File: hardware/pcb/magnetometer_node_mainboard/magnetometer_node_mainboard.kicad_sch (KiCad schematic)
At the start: 0 parts

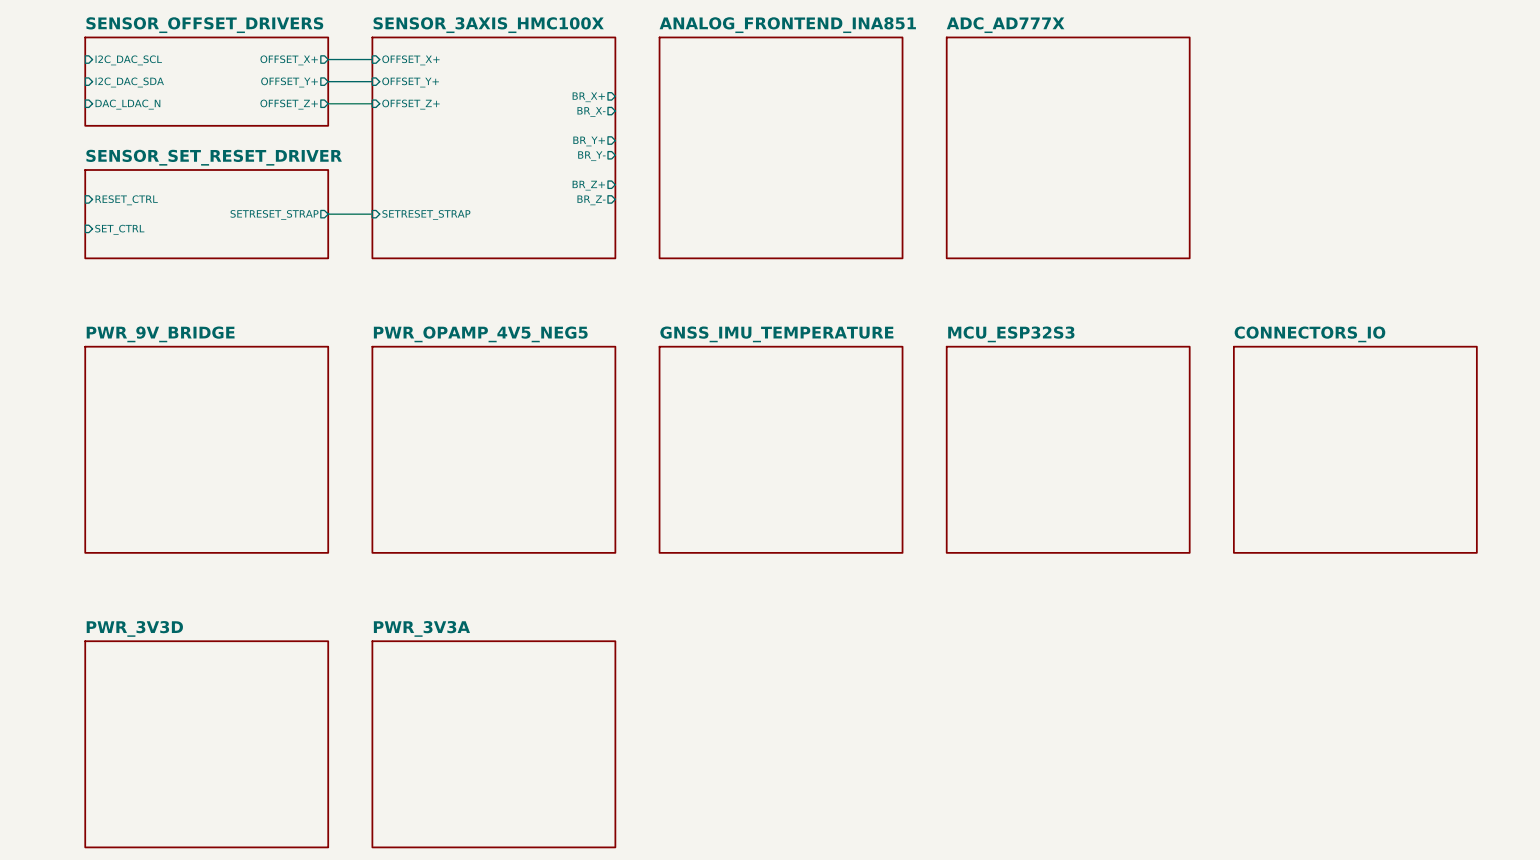
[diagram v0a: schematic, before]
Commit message: first code for the v1
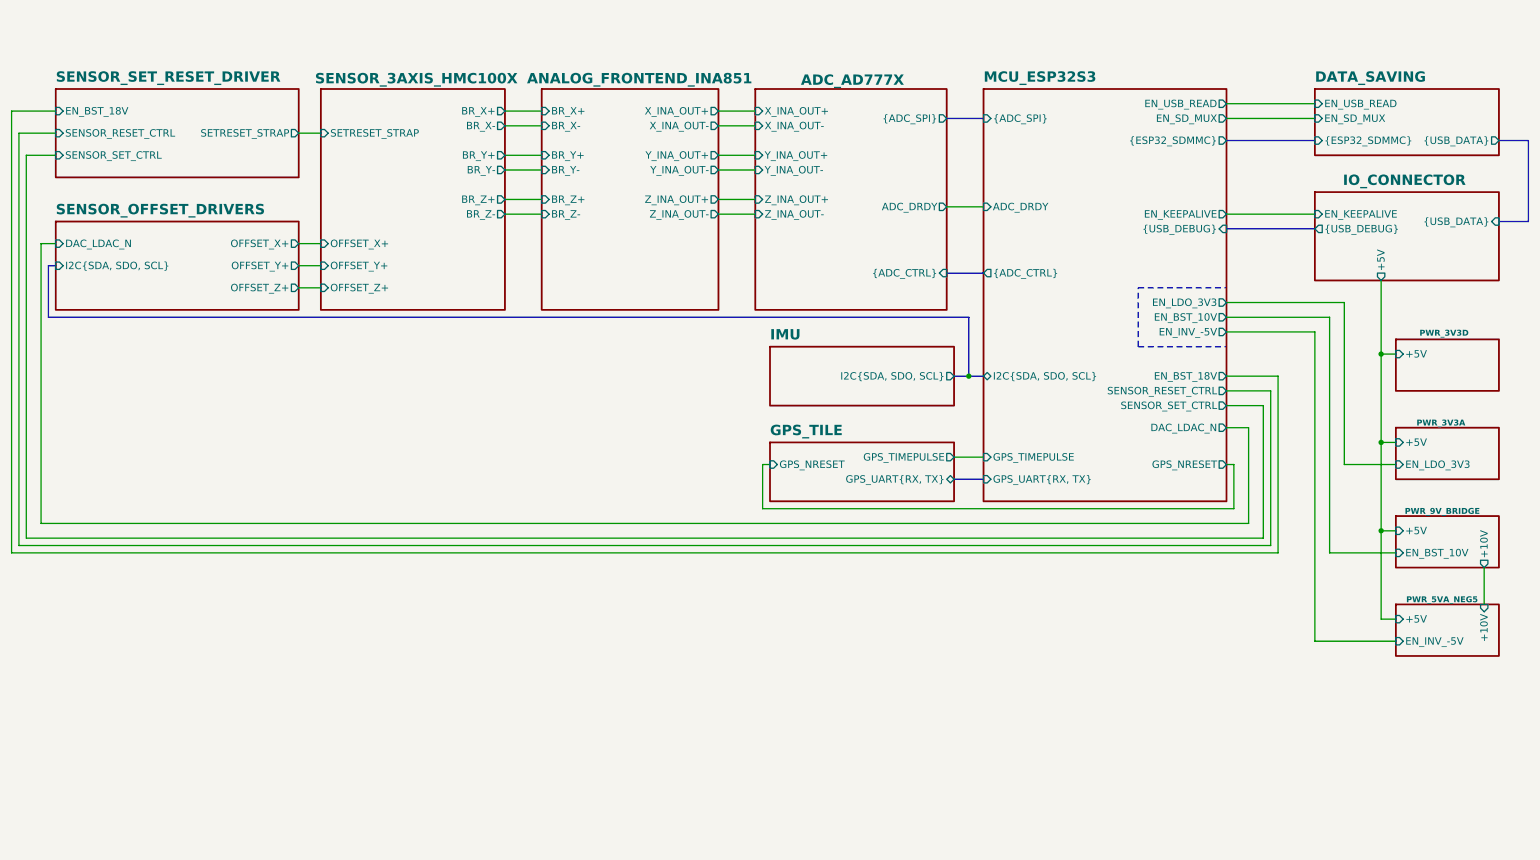
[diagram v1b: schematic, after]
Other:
- sheet CONNECTORS_IO renamed IO_CONNECTOR
- sheet GNSS_IMU_TEMPERATURE renamed IMU
- sheet PWR_OPAMP_4V5_NEG5 renamed PWR_5VA_NEG5
- added sheet DATA_SAVING (schematics/sd_card_saving_usb_to_pc.kicad_sch)
- added sheet GPS_TILE (schematics/GPS_tile.kicad_sch)
- sheet ADC_AD777X ports: added ADC_DRDY, X_INA_OUT+, X_INA_OUT-, Y_INA_OUT+, Y_INA_OUT-, Z_INA_OUT+, Z_INA_OUT-, {ADC_CTRL}, {ADC_SPI}; removed none
- sheet ANALOG_FRONTEND_INA851 ports: added BR_X+, BR_X-, BR_Y+, BR_Y-, BR_Z+, BR_Z-, X_INA_OUT+, X_INA_OUT-, Y_INA_OUT+, Y_INA_OUT-, Z_INA_OUT+, Z_INA_OUT-; removed none
- sheet IMU: file schematics/gnss_imu.kicad_sch -> schematics/imu.kicad_sch
- sheet IMU ports: added I2C{SDA, SDO, SCL}; removed none
- sheet IO_CONNECTOR ports: added +5V, EN_KEEPALIVE, {USB_DATA}, {USB_DEBUG}; removed none
- sheet MCU_ESP32S3 ports: added ADC_DRDY, DAC_LDAC_N, EN_BST_10V, EN_BST_18V, EN_INV_-5V, EN_KEEPALIVE, EN_LDO_3V3, EN_SD_MUX, EN_USB_READ, GPS_NRESET, GPS_TIMEPULSE, GPS_UART{RX, TX}, I2C{SDA, SDO, SCL}, SENSOR_RESET_CTRL, SENSOR_SET_CTRL, {ADC_CTRL}, {ADC_SPI}, {ESP32_SDMMC}, {USB_DEBUG}; removed none
- sheet PWR_3V3A ports: added +5V, EN_LDO_3V3; removed none
- sheet PWR_3V3D ports: added +5V; removed none
- sheet PWR_5VA_NEG5 ports: added +10V, +5V, EN_INV_-5V; removed none
- sheet PWR_9V_BRIDGE ports: added +10V, +5V, EN_BST_10V; removed none
- sheet SENSOR_OFFSET_DRIVERS ports: added I2C{SDA, SDO, SCL}; removed I2C_DAC_SCL, I2C_DAC_SDA
- sheet SENSOR_SET_RESET_DRIVER ports: added EN_BST_18V, SENSOR_RESET_CTRL, SENSOR_SET_CTRL; removed RESET_CTRL, SET_CTRL
